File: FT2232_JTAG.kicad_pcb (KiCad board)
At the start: 2 copper layers, 36.6 x 24 mm, 39 parts, among them J1 USB_C_Receptacle_USB2.0_16P, J2 Conn_01x09, J3 Conn_01x06, U1 FT2232HQ, U2 93LCxxB, U3 MCP1700x-330xxTT, Y1 12.000 MHz

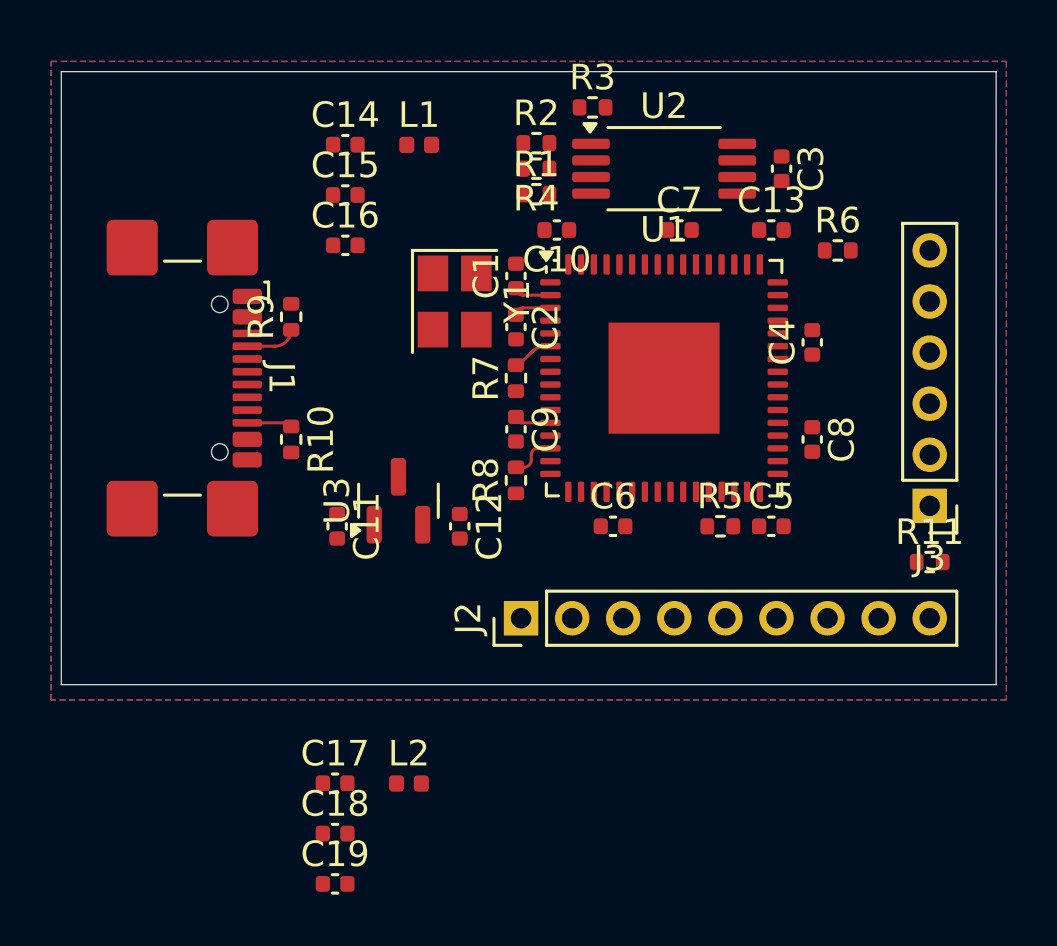
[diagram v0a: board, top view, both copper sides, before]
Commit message: wip
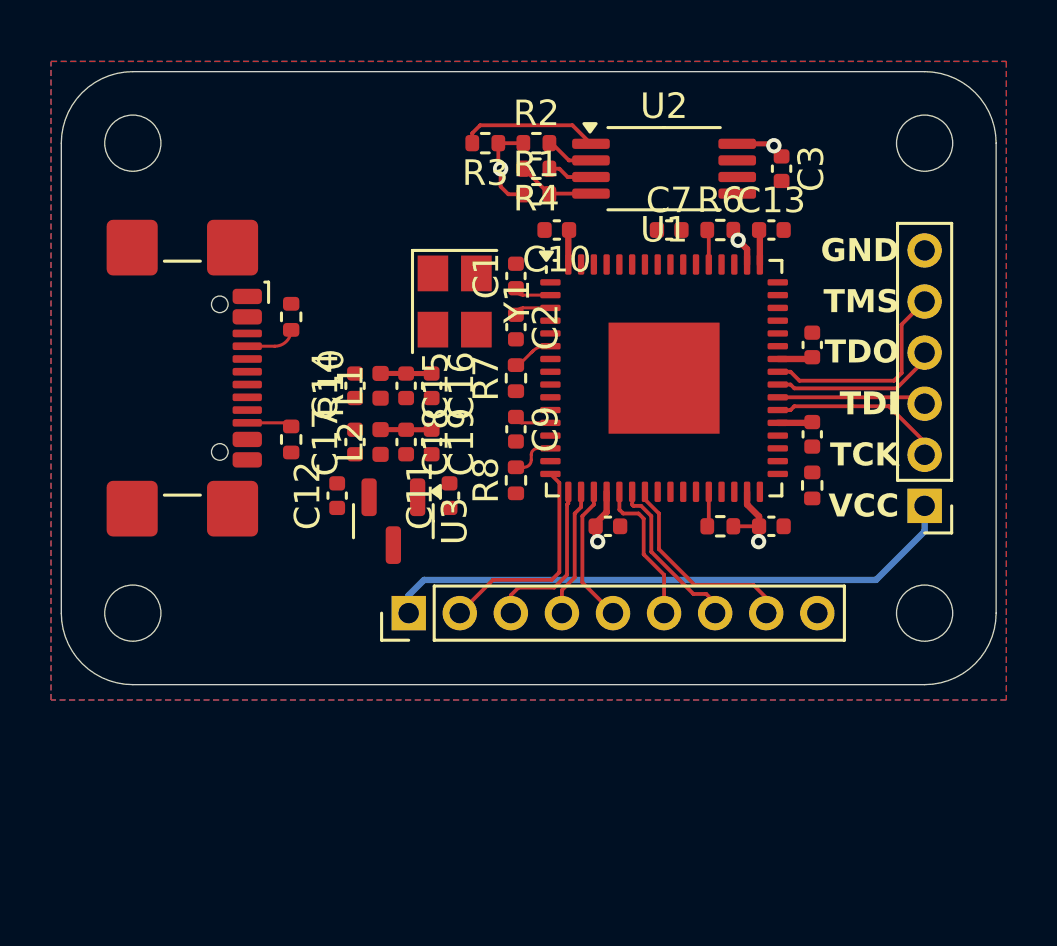
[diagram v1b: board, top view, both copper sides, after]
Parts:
- added H1: MountingHole, MountingHole:MountingHole_2.2mm_M2_ISO14580, F.Cu at (74.2, 90.8)
- added H2: MountingHole, MountingHole:MountingHole_2.2mm_M2_ISO14580, F.Cu at (105.2, 109.2)
- added H3: MountingHole, MountingHole:MountingHole_2.2mm_M2_ISO14580, F.Cu at (74.2, 109.2)
- added H4: MountingHole, MountingHole:MountingHole_2.2mm_M2_ISO14580, F.Cu at (105.2, 90.8)
- moved C19 17.7 mm to (85.9, 102.5), turned to -90 degrees
- moved C18 15.6 mm to (84.9, 102.5), turned to -90 degrees
- moved L2 13.4 mm to (83.9, 102.5), turned to 90 degrees
- moved C17 13.4 mm to (82.9, 102.5), turned to 90 degrees
- moved L1 9.55 mm to (83.9, 100.3), turned to 90 degrees
- moved C14 9.45 mm to (82.9, 100.3), turned to 90 degrees
- moved C15 7.84 mm to (84.9, 100.3), turned to -90 degrees
- moved C16 6.46 mm to (85.9, 100.3), turned to -90 degrees
- moved R11 5.49 mm to (100.8, 104.2), turned to -90 degrees
- moved C12 4.95 mm to (82.2, 104.6), turned to 90 degrees
- moved R6 4.67 mm to (97.2, 94.2)
- moved C11 4.56 mm to (86.6, 104.6), turned to 90 degrees
- moved R3 4.43 mm to (88.0, 90.8), turned to 180 degrees
- moved J2 4.40 mm to (85.0, 109.2)
- moved U3 0.82 mm to (84.4, 105.6), turned to -90 degrees
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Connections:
- net Net-(U1-DM) renamed /D-
- net Net-(U1-DP) renamed /D+
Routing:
- net +3.3VP: track 0.00 -> 22.9 mm
- net +3.3V: track 0.00 -> 13.9 mm, vias 0 -> 5
- net /CLK: track 0.00 -> 8.56 mm
- net /TMS: track 0.00 -> 8.29 mm
- net /HOLD: track 0.00 -> 8.06 mm
- net /TCK: track 0.00 -> 6.89 mm
- net /TDO: track 0.00 -> 6.57 mm
- net /CDONE: track 0.00 -> 6.56 mm
- net /MOSI: track 0.00 -> 6.50 mm
- net /TDI: track 0.00 -> 5.85 mm
- net /CRESET_B: track 0.00 -> 5.83 mm
- net Net-(U1-EECS): track 0.00 -> 5.47 mm
- net /SS: track 0.00 -> 5.43 mm
- net /MISO: track 0.00 -> 5.06 mm
- net +1V8: track 1.47 -> 5.56 mm
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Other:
- outline, holes or cut-outs redrawn
- board text added: "GND"
- board text added: "TCK"
- board text added: "TDI"
- board text added: "TDO"
- board text added: "TMS"
- board text added: "VCC"
